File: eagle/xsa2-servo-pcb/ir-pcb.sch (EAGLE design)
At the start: 62 parts, among them IC1 ATMEGA328P-AU, IC10 SK6812_SIDE, IC11 SK6812_SIDE, IC12 SK6812_SIDE, IC13 SK6812_SIDE, IC14 SK6812_SIDE, IC15 SK6812_SIDE, IC16 SK6812_SIDE, IC17 SK6812_SIDE, IC18 SK6812_SIDE, IC19 SK6812_SIDE, IC2 PL-IRM0101, IC3 PL-IRM0101, IC4 PL-IRM0101, IC5 PL-IRM0101, IC6 PL-IRM0101, IC7 PL-IRM0101, IC8 SK6812_SIDE, IC9 SK6812_SIDE, Q1 IRLML6402, Q2 IRFML8244, Q3 IRFML8244, Q4 IRFML8244, Q5 8MHz, Q6 IRFML8244

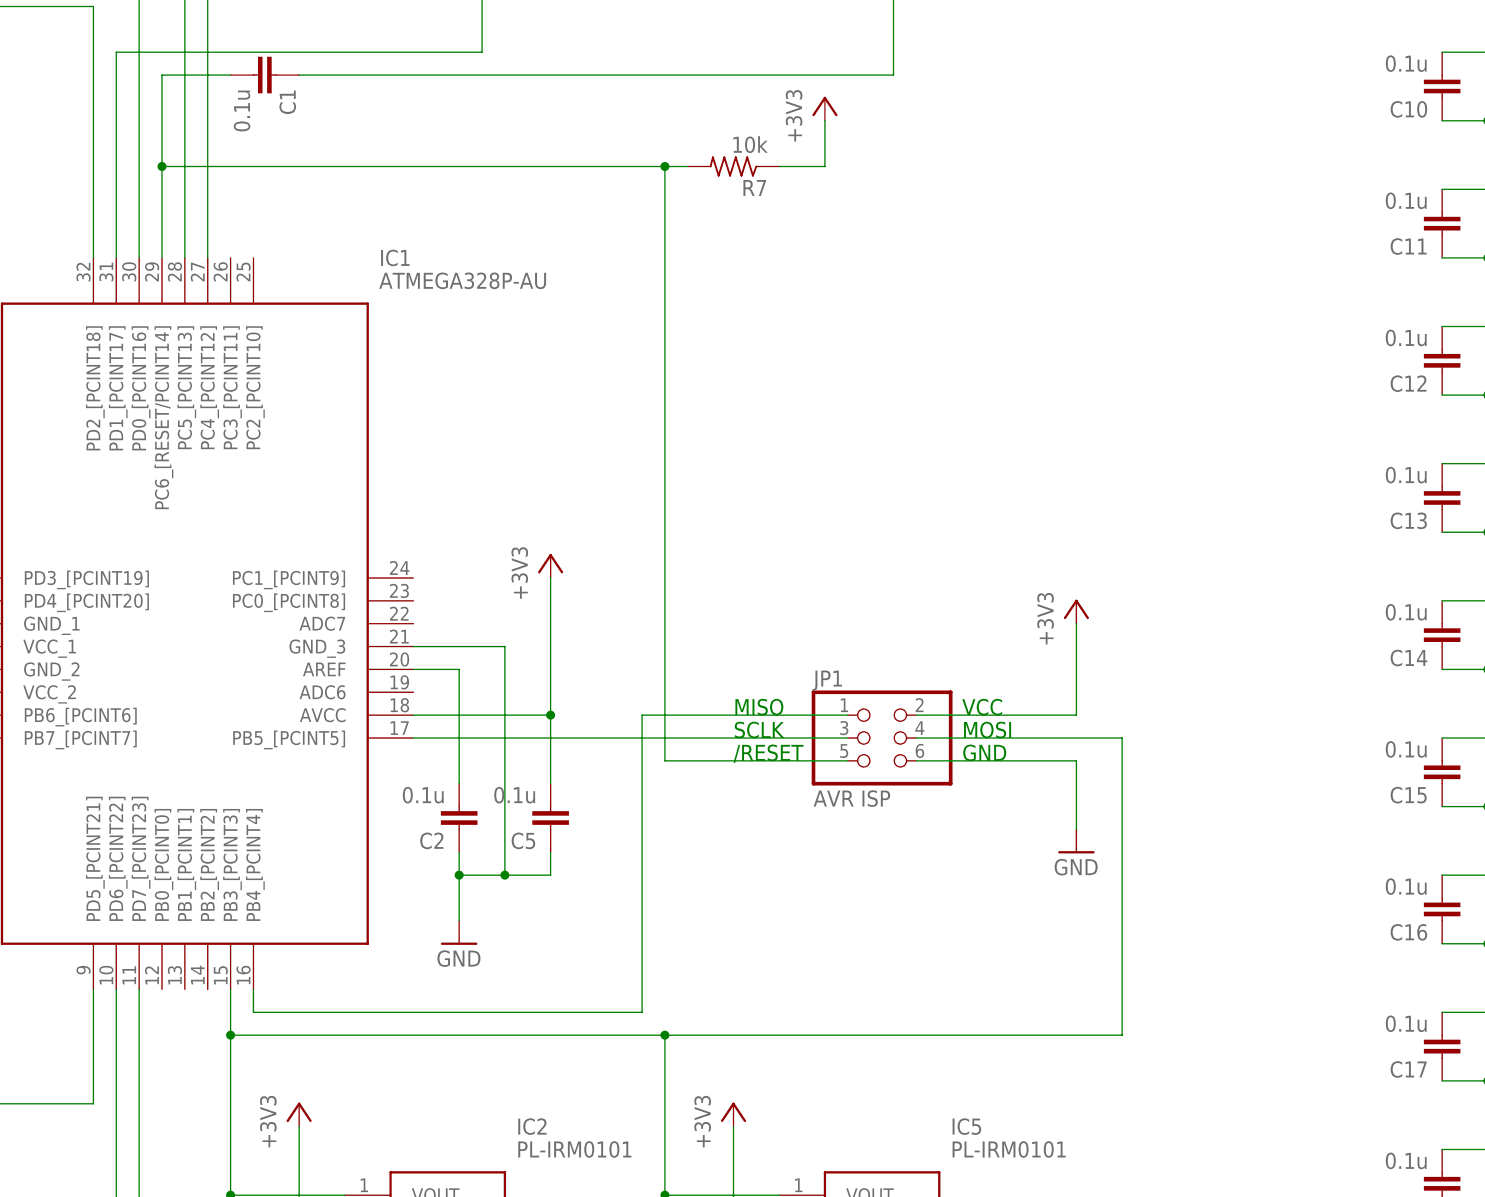
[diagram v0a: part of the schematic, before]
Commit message: [eagle] サーボ基板完成
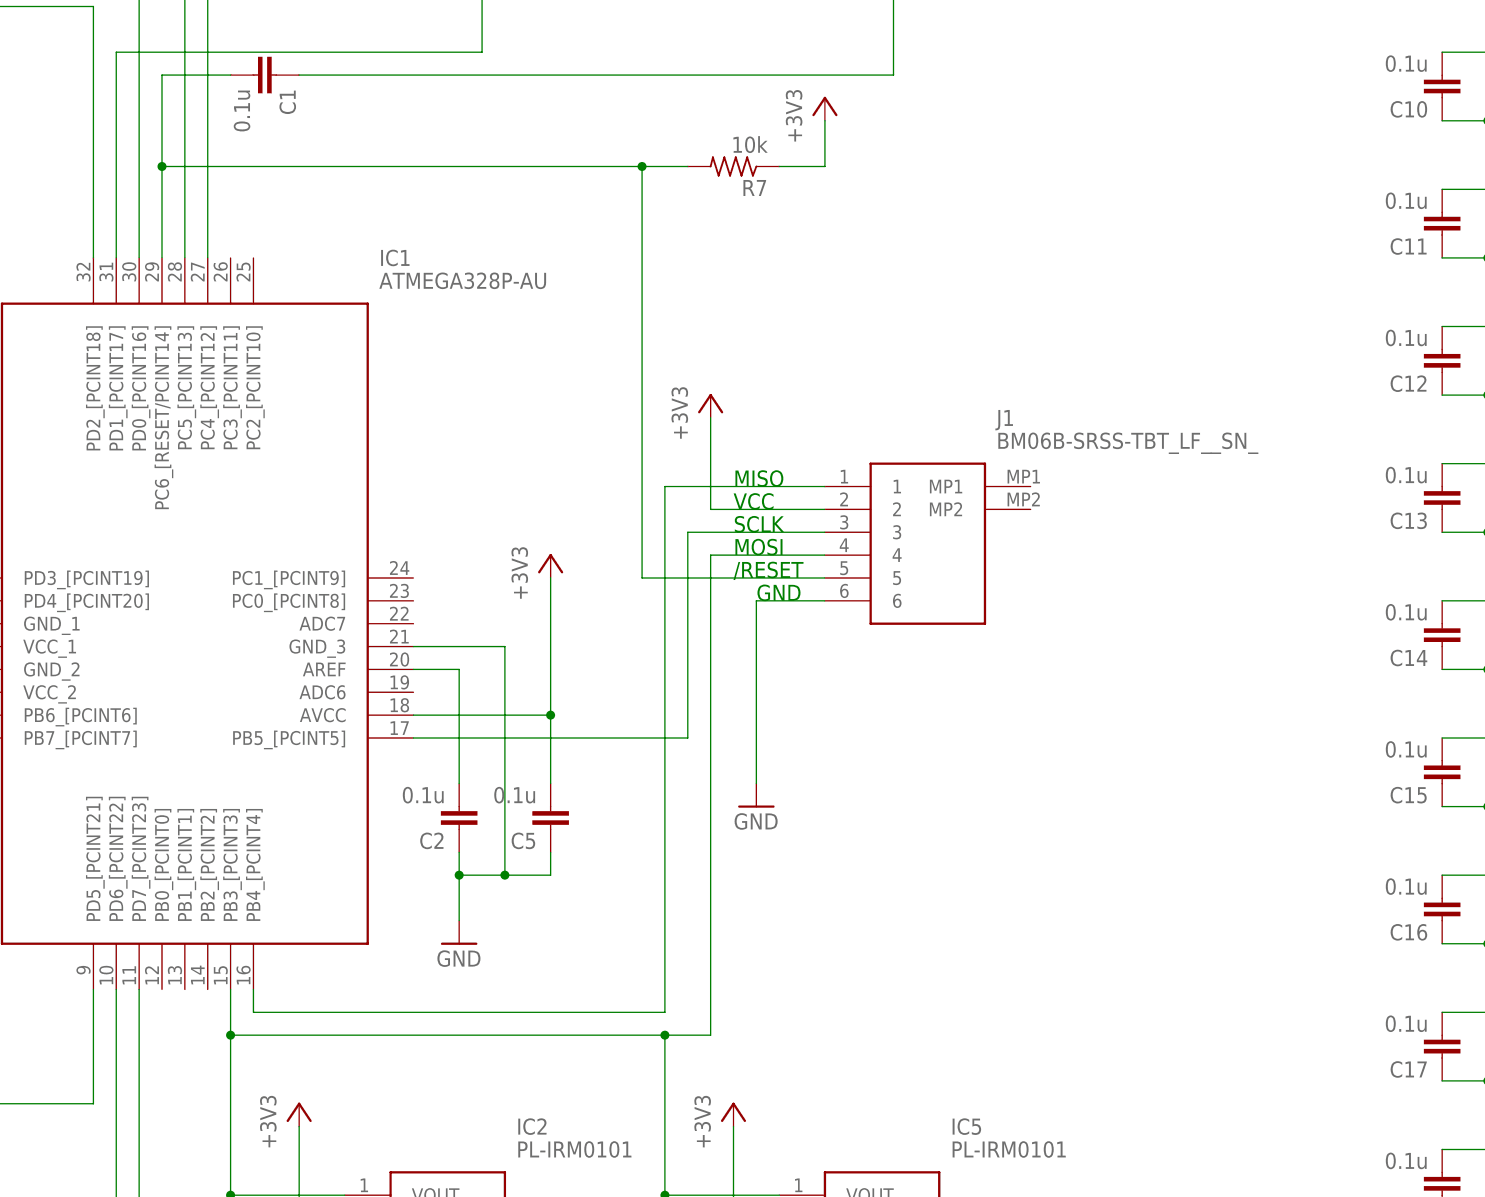
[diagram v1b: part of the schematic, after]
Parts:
- removed JP1: AVR ISP, pinhead:PINHD-2X3
- added J1: BM06B-SRSS-TBT_LF__SN_, SamacSys_Parts:BM06B-SRSS-TBT_LF__SN_
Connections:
- net +3V3: now also J1.2; no longer JP1.2
- net GND: now also J1.6; no longer JP1.6
- net N$1: now also J1.1; no longer JP1.1
- net N$25: now also J1.5; no longer JP1.5
- net N$41: now also J1.4; no longer JP1.4
- net N$5: now also J1.3; no longer JP1.3
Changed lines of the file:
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@@
 <part name="LED5" library="SamacSys_Parts" library_urn="urn:adsk.eagle:library:36791783" deviceset="OSI5FU5111C-40" device="" package3d_urn="urn:adsk.eagle:package:36791786/1"/>
 <part name="LED6" library="SamacSys_Parts" library_urn="urn:adsk.eagle:library:36791783" deviceset="OSI5FU5111C-40" device="" package3d_urn="urn:adsk.eagle:package:36791786/1"/>
-<part name="JP1" library="pinhead" library_urn="urn:adsk.eagle:library:325" deviceset="PINHD-2X3" device="" package3d_urn="urn:adsk.eagle:package:22462/2" value="AVR ISP"/>
 <part name="JP3" library="pinhead" library_urn="urn:adsk.eagle:library:325" deviceset="PINHD-2X7" device="" package3d_urn="urn:adsk.eagle:package:22478/2" value="Stacking Connector"/>
 <part name="+3V1" library="supply1" library_urn="urn:adsk.eagle:library:371" deviceset="+3V3" device=""/>
@@
 <part name="R15" library="rcl" library_urn="urn:adsk.eagle:library:334" deviceset="R-US_" device="R2512W" package3d_urn="urn:adsk.eagle:package:23565/2" value="10"/>
 <part name="R2" library="rcl" library_urn="urn:adsk.eagle:library:334" deviceset="R-US_" device="R2512W" package3d_urn="urn:adsk.eagle:package:23565/2" value="39"/>
+<part name="J1" library="SamacSys_Parts" deviceset="BM06B-SRSS-TBT_LF__SN_" device=""/>
 </parts>
 <sheets>
@@
 <text x="0" y="83.82" size="1.778" layer="91">RXD</text>
 <text x="35.56" y="83.82" size="1.778" layer="91">DTR</text>
-<text x="25.4" y="-20.32" size="1.778" layer="91">MISO</text>
-<text x="50.8" y="-20.32" size="1.778" layer="91">VCC</text>
-<text x="25.4" y="-22.86" size="1.778" layer="91">SCLK</text>
-<text x="50.8" y="-22.86" size="1.778" layer="91">MOSI</text>
-<text x="25.4" y="-25.4" size="1.778" layer="91">/RESET</text>
-<text x="50.8" y="-25.4" size="1.778" layer="91">GND</text>
+<text x="25.4" y="5.08" size="1.778" layer="91">MISO</text>
+<text x="25.4" y="2.54" size="1.778" layer="91">VCC</text>
+<text x="25.4" y="0" size="1.778" layer="91">SCLK</text>
+<text x="25.4" y="-2.54" size="1.778" layer="91">MOSI</text>
+<text x="25.4" y="-5.08" size="1.778" layer="91">/RESET</text>
+<text x="27.94" y="-7.62" size="1.778" layer="91">GND</text>
 <text x="-27.94" y="88.9" size="1.778" layer="91">GND</text>
 <text x="-50.8" y="76.2" size="1.778" layer="91">+5V</text>
@@
 <attribute name="VALUE" x="-133.35" y="-17.78" size="1.778" layer="96" rot="R90"/>
 </instance>
-<instance part="JP1" gate="A" x="40.64" y="-22.86" smashed="yes">
-<attribute name="NAME" x="34.29" y="-17.145" size="1.778" layer="95"/>
-<attribute name="VALUE" x="34.29" y="-30.48" size="1.778" layer="96"/>
-</instance>
 <instance part="JP3" gate="A" x="-38.1" y="81.28" smashed="yes">
 <attribute name="NAME" x="-44.45" y="89.535" size="1.778" layer="95"/>
 <attribute name="VALUE" x="-44.45" y="68.58" size="1.778" layer="96"/>
 </instance>
-<instance part="+3V1" gate="G$1" x="63.5" y="-7.62" smashed="yes">
-<attribute name="VALUE" x="60.96" y="-12.7" size="1.778" layer="96" rot="R90"/>
-</instance>
-<instance part="GND1" gate="1" x="63.5" y="-35.56" smashed="yes">
-<attribute name="VALUE" x="60.96" y="-38.1" size="1.778" layer="96"/>
+<instance part="+3V1" gate="G$1" x="22.86" y="15.24" smashed="yes">
+<attribute name="VALUE" x="20.32" y="10.16" size="1.778" layer="96" rot="R90"/>
+</instance>
+<instance part="GND1" gate="1" x="27.94" y="-30.48" smashed="yes">
+<attribute name="VALUE" x="25.4" y="-33.02" size="1.778" layer="96"/>
 </instance>
 <instance part="+3V3" gate="G$1" x="25.4" y="-63.5" smashed="yes">
@@
 <attribute name="NAME" x="-108.1786" y="-46.99" size="1.778" layer="95" rot="R90"/>
 <attribute name="VALUE" x="-103.378" y="-46.99" size="1.778" layer="96" rot="R90"/>
+</instance>
+<instance part="J1" gate="G$1" x="35.56" y="5.08" smashed="yes">
+<attribute name="NAME" x="54.61" y="12.7" size="1.778" layer="95" align="center-left"/>
+<attribute name="VALUE" x="54.61" y="10.16" size="1.778" layer="96" align="center-left"/>
 </instance>
 </instances>
@@
 <segment>
 <pinref part="IC1" gate="G$1" pin="PB5_[PCINT5]"/>
-<wire x1="-10.16" y1="-22.86" x2="38.1" y2="-22.86" width="0.1524" layer="91"/>
-<pinref part="JP1" gate="A" pin="3"/>
+<wire x1="-10.16" y1="-22.86" x2="20.32" y2="-22.86" width="0.1524" layer="91"/>
+<wire x1="20.32" y1="-22.86" x2="20.32" y2="0" width="0.1524" layer="91"/>
+<wire x1="20.32" y1="0" x2="35.56" y2="0" width="0.1524" layer="91"/>
+<pinref part="J1" gate="G$1" pin="3"/>
 </segment>
 </net>
@@
 <segment>
 <pinref part="IC1" gate="G$1" pin="PB4_[PCINT4]"/>
-<pinref part="JP1" gate="A" pin="1"/>
 <wire x1="-27.94" y1="-50.8" x2="-27.94" y2="-53.34" width="0.1524" layer="91"/>
-<wire x1="-27.94" y1="-53.34" x2="15.24" y2="-53.34" width="0.1524" layer="91"/>
-<wire x1="15.24" y1="-53.34" x2="15.24" y2="-20.32" width="0.1524" layer="91"/>
-<wire x1="15.24" y1="-20.32" x2="38.1" y2="-20.32" width="0.1524" layer="91"/>
+<wire x1="-27.94" y1="-53.34" x2="17.78" y2="-53.34" width="0.1524" layer="91"/>
+<wire x1="17.78" y1="-53.34" x2="17.78" y2="5.08" width="0.1524" layer="91"/>
+<wire x1="17.78" y1="5.08" x2="35.56" y2="5.08" width="0.1524" layer="91"/>
+<pinref part="J1" gate="G$1" pin="1"/>
 </segment>
 </net>
@@
 <segment>
 <pinref part="+3V1" gate="G$1" pin="+3V3"/>
-<pinref part="JP1" gate="A" pin="2"/>
-<wire x1="63.5" y1="-10.16" x2="63.5" y2="-20.32" width="0.1524" layer="91"/>
-<wire x1="63.5" y1="-20.32" x2="45.72" y2="-20.32" width="0.1524" layer="91"/>
+<wire x1="22.86" y1="12.7" x2="22.86" y2="2.54" width="0.1524" layer="91"/>
+<wire x1="22.86" y1="2.54" x2="35.56" y2="2.54" width="0.1524" layer="91"/>
+<pinref part="J1" gate="G$1" pin="2"/>
 </segment>
 <segment>
@@
 <net name="GND" class="0">
 <segment>
-<pinref part="JP1" gate="A" pin="6"/>
-<wire x1="45.72" y1="-25.4" x2="63.5" y2="-25.4" width="0.1524" layer="91"/>
+<wire x1="35.56" y1="-7.62" x2="27.94" y2="-7.62" width="0.1524" layer="91"/>
 <pinref part="GND1" gate="1" pin="GND"/>
-<wire x1="63.5" y1="-25.4" x2="63.5" y2="-33.02" width="0.1524" layer="91"/>
+<wire x1="27.94" y1="-7.62" x2="27.94" y2="-27.94" width="0.1524" layer="91"/>
+<pinref part="J1" gate="G$1" pin="6"/>
 </segment>
 <segment>
@@
 <net name="N$25" class="0">
 <segment>
-<pinref part="JP1" gate="A" pin="5"/>
-<wire x1="38.1" y1="-25.4" x2="17.78" y2="-25.4" width="0.1524" layer="91"/>
+<wire x1="35.56" y1="-5.08" x2="15.24" y2="-5.08" width="0.1524" layer="91"/>
 <pinref part="IC1" gate="G$1" pin="PC6_[RESET/PCINT14]"/>
 <wire x1="-38.1" y1="50.8" x2="-38.1" y2="40.64" width="0.1524" layer="91"/>
@@
 <pinref part="C1" gate="G$1" pin="2"/>
 <wire x1="-30.48" y1="50.8" x2="-38.1" y2="50.8" width="0.1524" layer="91"/>
-<wire x1="17.78" y1="-25.4" x2="17.78" y2="40.64" width="0.1524" layer="91"/>
-<wire x1="17.78" y1="40.64" x2="-38.1" y2="40.64" width="0.1524" layer="91"/>
+<wire x1="15.24" y1="-5.08" x2="15.24" y2="40.64" width="0.1524" layer="91"/>
+<wire x1="15.24" y1="40.64" x2="-38.1" y2="40.64" width="0.1524" layer="91"/>
 <junction x="-38.1" y="40.64"/>
 <pinref part="R7" gate="G$1" pin="2"/>
-<wire x1="17.78" y1="40.64" x2="20.32" y2="40.64" width="0.1524" layer="91"/>
-<junction x="17.78" y="40.64"/>
+<wire x1="15.24" y1="40.64" x2="20.32" y2="40.64" width="0.1524" layer="91"/>
+<junction x="15.24" y="40.64"/>
+<pinref part="J1" gate="G$1" pin="5"/>
 </segment>
 </net>
@@
 <wire x1="-30.48" y1="-50.8" x2="-30.48" y2="-55.88" width="0.1524" layer="91"/>
 <wire x1="-30.48" y1="-55.88" x2="17.78" y2="-55.88" width="0.1524" layer="91"/>
-<wire x1="17.78" y1="-55.88" x2="68.58" y2="-55.88" width="0.1524" layer="91"/>
-<wire x1="68.58" y1="-55.88" x2="68.58" y2="-22.86" width="0.1524" layer="91"/>
-<pinref part="JP1" gate="A" pin="4"/>
-<wire x1="68.58" y1="-22.86" x2="45.72" y2="-22.86" width="0.1524" layer="91"/>
+<wire x1="17.78" y1="-55.88" x2="22.86" y2="-55.88" width="0.1524" layer="91"/>
+<wire x1="22.86" y1="-55.88" x2="22.86" y2="-2.54" width="0.1524" layer="91"/>
+<wire x1="22.86" y1="-2.54" x2="35.56" y2="-2.54" width="0.1524" layer="91"/>
 <junction x="-30.48" y="-55.88"/>
 <junction x="17.78" y="-55.88"/>
-</segment>
-</net>
+<pinref part="J1" gate="G$1" pin="4"/>
+</segment>
+</net>
